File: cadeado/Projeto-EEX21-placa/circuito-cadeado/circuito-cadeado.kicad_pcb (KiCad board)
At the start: 2 copper layers, 100.6 x 53.8 mm, 15 parts

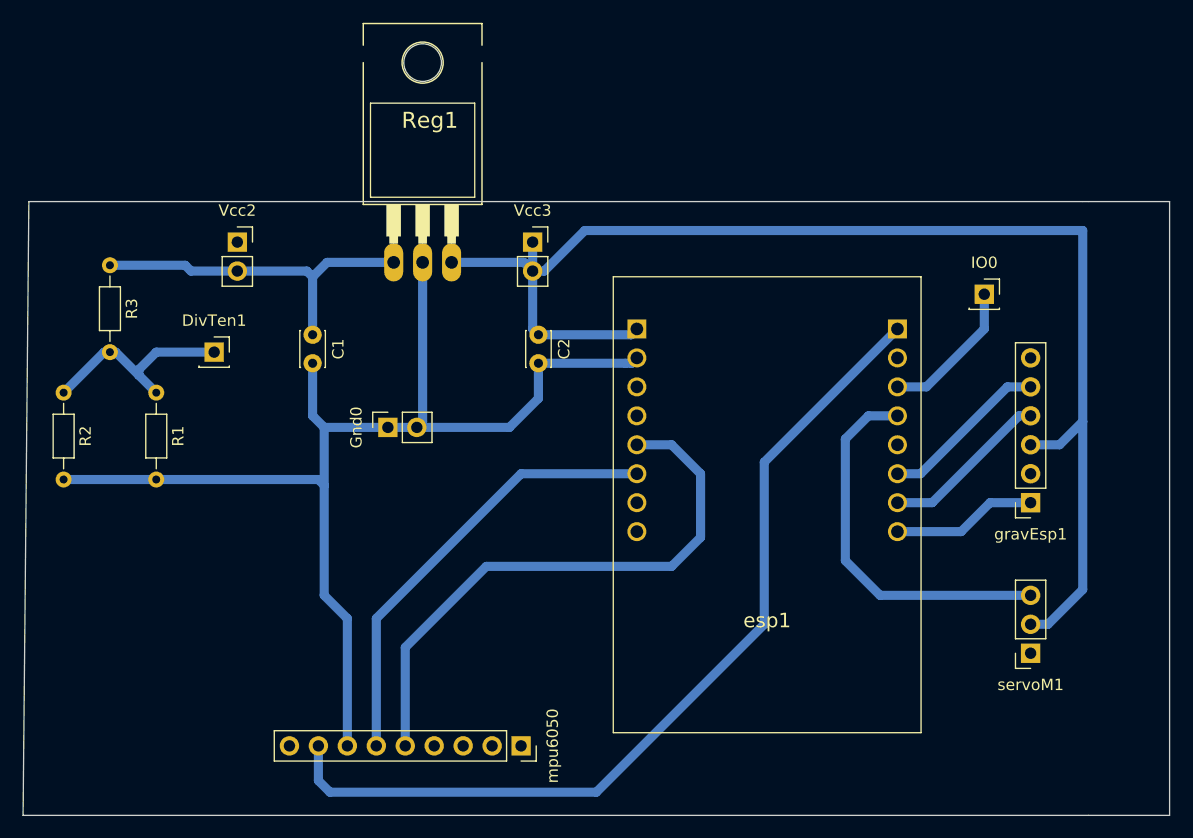
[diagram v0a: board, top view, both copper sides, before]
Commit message: atualização circuito impresso v1.1
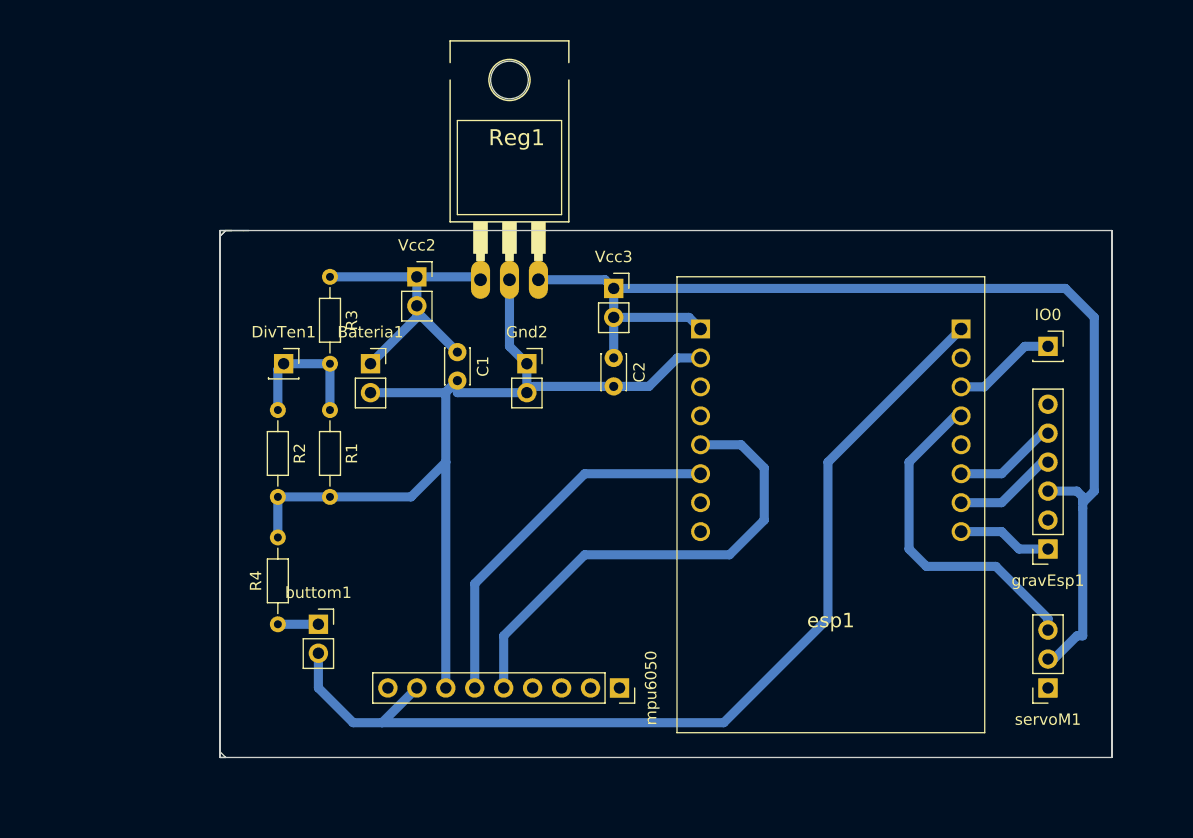
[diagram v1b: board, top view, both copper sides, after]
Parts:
- added Gnd2: 0, Connector_PinSocket_2.54mm:PinSocket_1x02_P2.54mm_Vertical, F.Cu at (131.6, 86.9)
- added R4: 10K, Resistor_THT:R_Axial_DIN0204_L3.6mm_D1.6mm_P7.62mm_Horizontal, F.Cu at (109.7, 109.7)
- added buttom1: 0, Connector_PinSocket_2.54mm:PinSocket_1x02_P2.54mm_Vertical, F.Cu at (113.3, 109.7)
- moved R3 19.3 mm to (114.3, 79.2)
- moved R2 18.9 mm to (109.7, 90.9)
- moved Vcc2 16.0 mm to (121.9, 79.2)
- moved R1 15.3 mm to (114.3, 90.9)
- moved C1 12.8 mm to (125.5, 85.9)
- moved mpu6050 10.0 mm to (139.7, 115.3)
- moved Vcc3 8.19 mm to (139.2, 80.3)
- moved Reg1 7.77 mm to (130.0, 73.2)
- moved IO0 7.22 mm to (177.3, 85.3)
- moved C2 6.91 mm to (139.2, 86.4)
- moved DivTen1 6.18 mm to (110.2, 86.9)
- moved Bateria1 5.79 mm to (117.9, 86.9), turned to 0 degrees
- moved esp1 5.59 mm to (146.8, 101.6)
- moved gravEsp1 4.34 mm to (177.3, 103.1)
- moved servoM1 3.41 mm to (177.3, 115.3)
- renumbered Gnd0 to Bateria1
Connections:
- Bateria1 pad 1: GNDREF -> +9V
- servoM1 pad 1: Net-(esp1-Pad1) -> Net-(esp1-Pad5)
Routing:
- net Net-(C2-Pad1): track 117.8 -> 100.3 mm
- net GNDREF: track 105.0 -> 89.2 mm
- net Net-(esp1-Pad4): track 50.8 -> 42.6 mm
- net Net-(buttom1-Pad2): track 79.4 -> 87.4 mm
- net Net-(DivTen1-Pad1): track 18.8 -> 12.4 mm
- net Net-(esp1-Pad3): track 39.3 -> 33.0 mm
- net Net-(esp1-Pad15): track 14.8 -> 9.09 mm
- net Net-(esp1-Pad14): track 14.8 -> 9.09 mm
- net Net-(esp1-Pad16): track 12.7 -> 8.25 mm
- net Net-(esp1-Pad12): track 33.6 -> 29.6 mm
- net Net-(IO0-Pad1): track 12.8 -> 9.09 mm
- net Net-(R4-Pad1): track 0.00 -> 3.56 mm
- net +9V: track 31.6 -> 28.2 mm
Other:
- board size 100.6 x 53.8 mm -> 78.2 x 46.2 mm
